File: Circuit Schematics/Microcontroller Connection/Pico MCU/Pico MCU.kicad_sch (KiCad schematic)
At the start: 3 parts

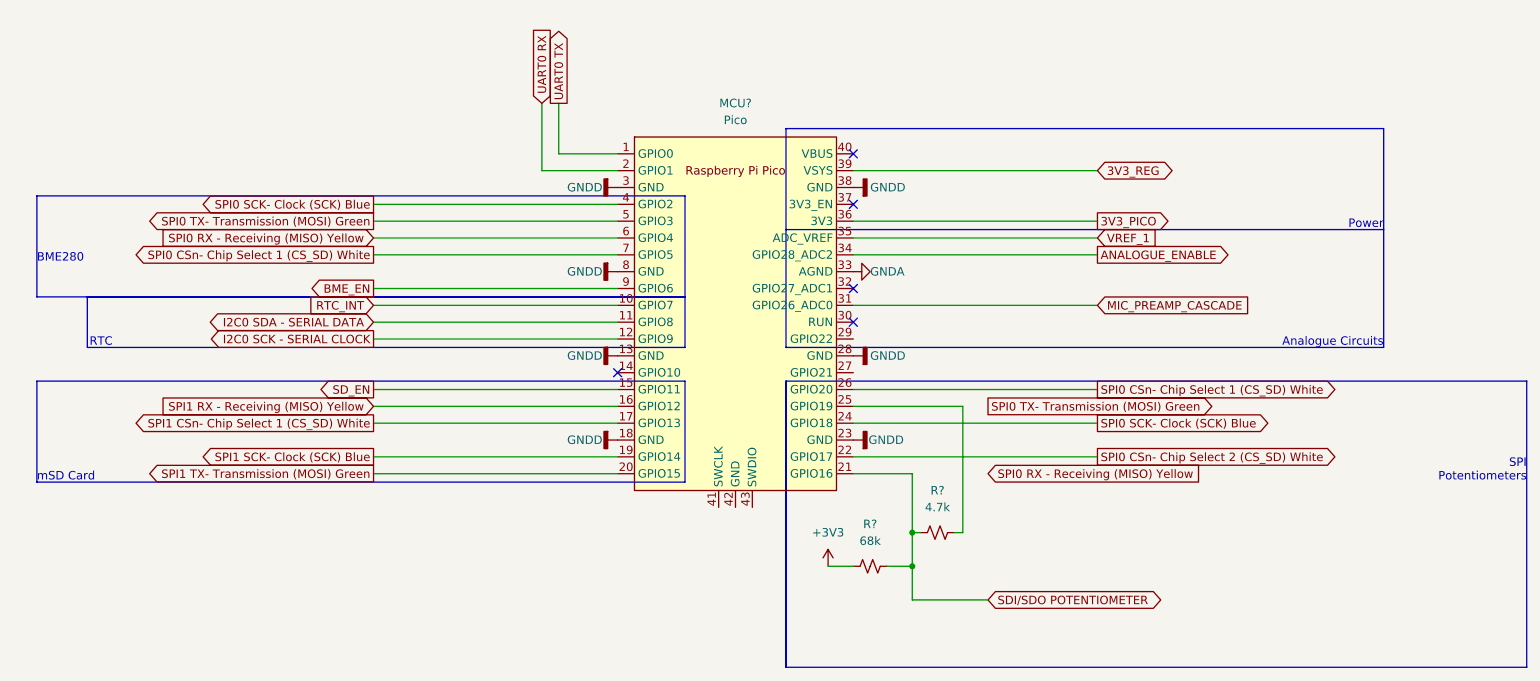
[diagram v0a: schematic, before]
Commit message: Whole boatload of changes
Latest.
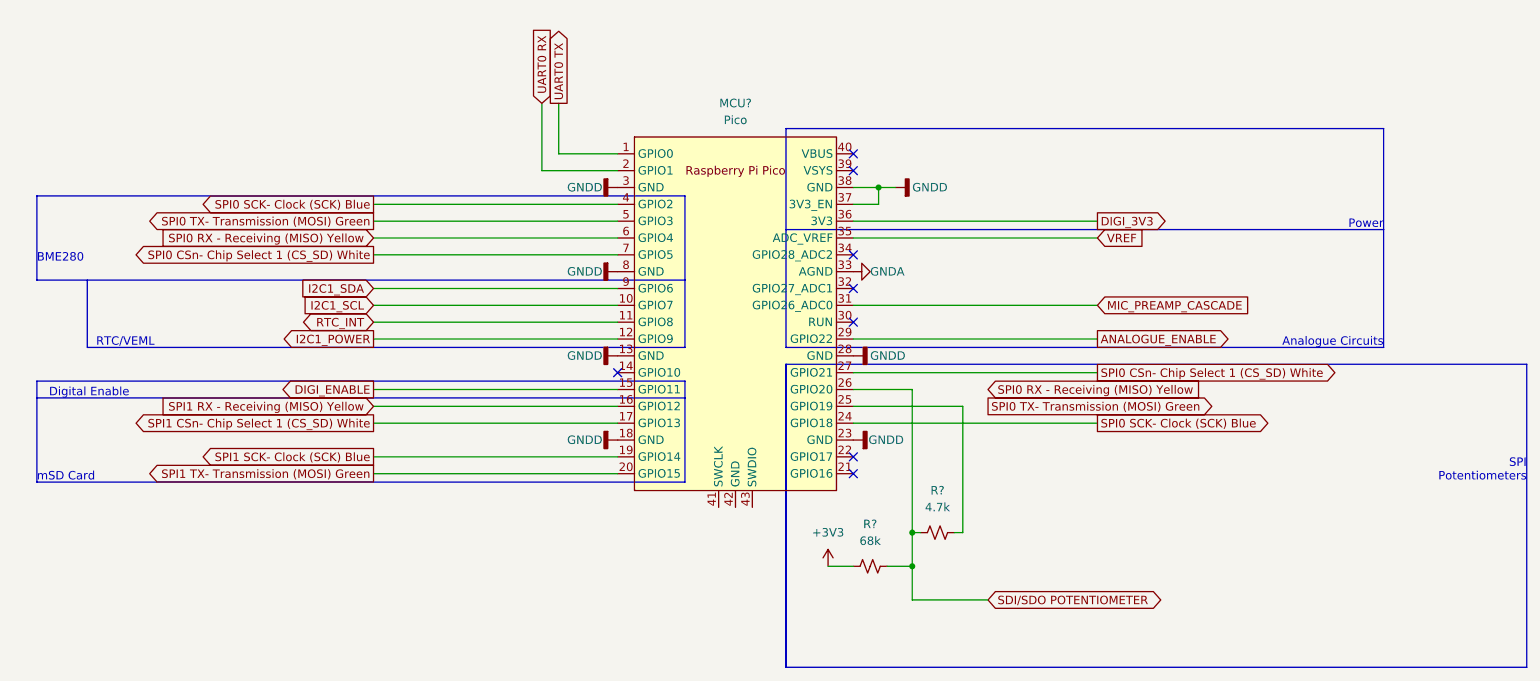
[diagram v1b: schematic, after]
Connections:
- net I2C0 SDA - SERIAL DATA  is gone; now on net RTC_INT: MCU?.11 (GPIO8)
- net ANALOGUE_ENABLE: now also MCU?.29 (GPIO22); no longer MCU?.34 (GPIO28_ADC2)
- net GNDD: now also MCU?.37 (3V3_EN)
- net RTC_INT: no longer MCU?.10 (GPIO7)
- net SDI/SDO POTENTIOMETER: now also MCU?.26 (GPIO20); no longer MCU?.21 (GPIO16)
- net SPI0 CSn- Chip Select 1 (CS_SD) White: now also MCU?.27 (GPIO21); no longer MCU?.26 (GPIO20)
- net 3V3_PICO renamed DIGI_3V3
- net 3V3_REG: no longer names the net of MCU?.39 (VSYS)
- net BME_EN renamed I2C1_SDA
- net I2C0 SCK - SERIAL CLOCK renamed I2C1_POWER
- net SD_EN renamed DIGI_ENABLE
- net SPI0 CSn- Chip Select 2 (CS_SD) White: no longer names the net of MCU?.22 (GPIO17)
- net VREF_1 renamed VREF
- new net I2C1_SCL: MCU?.10 (GPIO7)
- no-connect marks 5 -> 8
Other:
- note added: "Digital Enable"
- note added: "RTC/VEML"
- note removed: "RTC"
